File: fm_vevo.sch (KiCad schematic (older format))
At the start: 77 parts, among them J1 Bemenet, J2 RedPitaya_OSC, J3 12VDC, J4 RedPitaya_IN, J5 AudioJack2, Q1 mmbfj310, Q2 MMBT3904, Q3 MMBT3904, Q4 MMBT3904, Q5 MMBT3904, U1 LM358

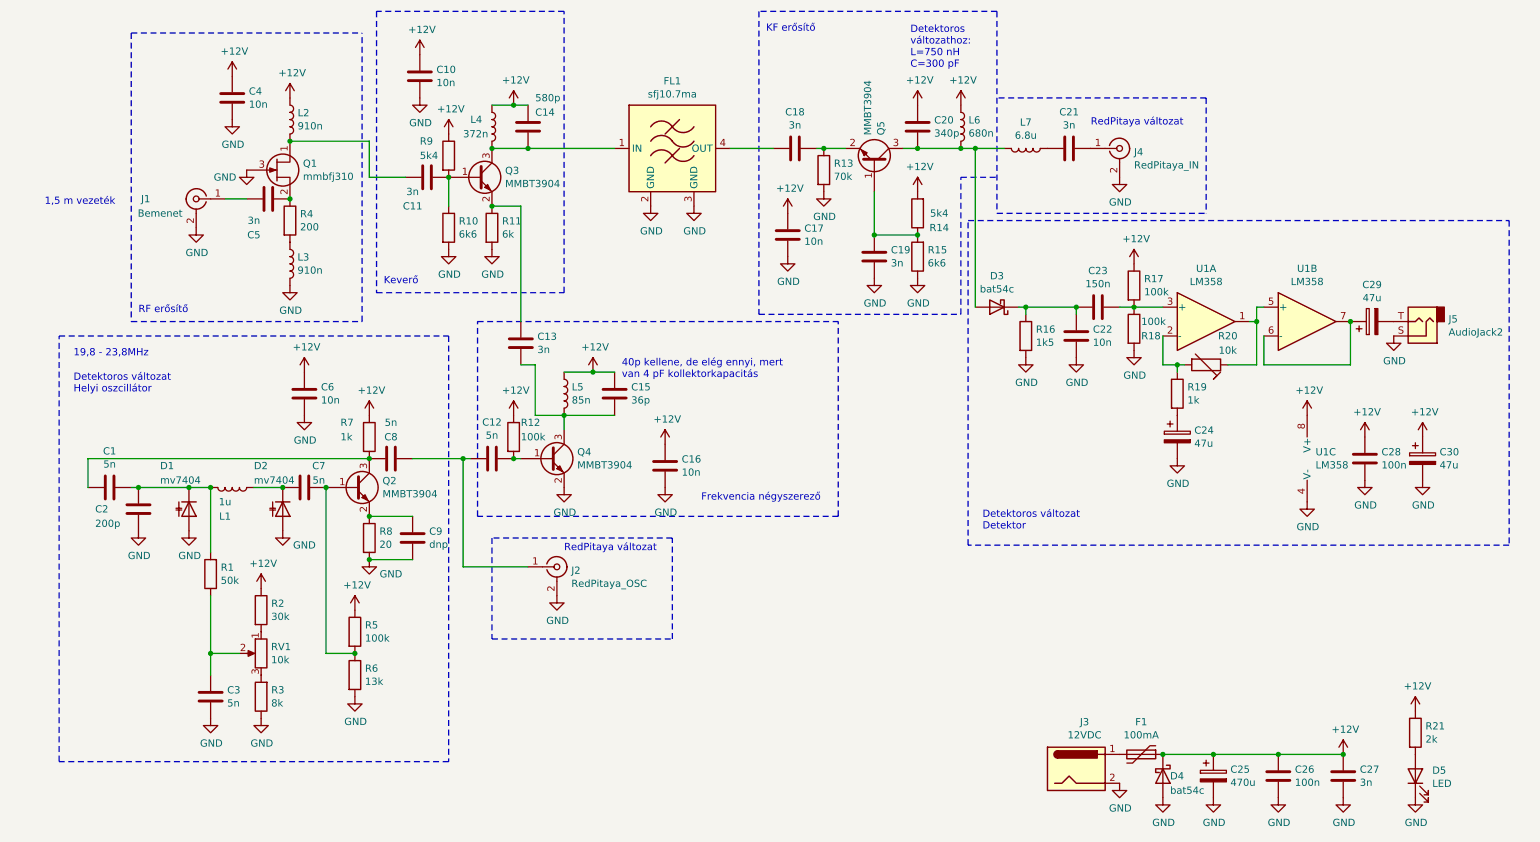
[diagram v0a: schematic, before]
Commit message: first sa612
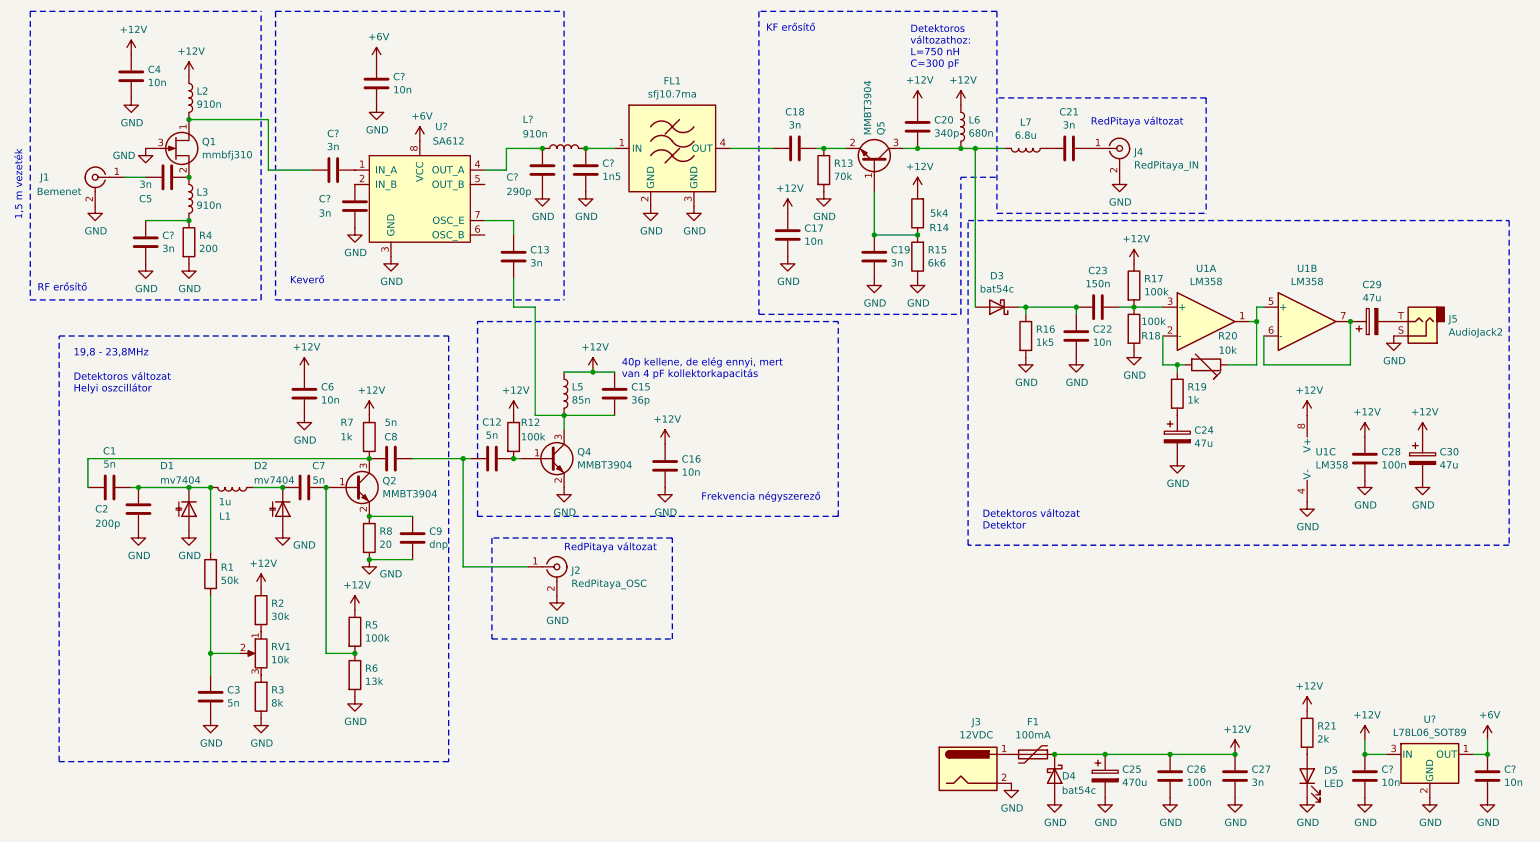
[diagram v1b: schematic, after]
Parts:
- removed C10: 10n, symbol Device:C
- removed C11: 3n, symbol Device:C
- removed C14: 580p, symbol Device:C
- removed L4: 372n, symbol Device:L
- removed Q3: MMBT3904, Package_TO_SOT_SMD:SOT-23, symbol Transistor_BJT:MMBT3904
- removed R10: 6k6, symbol Device:R
- removed R11: 6k, symbol Device:R
- removed R9: 5k4, symbol Device:R
- added C? (x3): 10n, symbol Device:C
- added C? (x3): 3n, symbol Device:C
- added C?: 290p, symbol Device:C
- added C?: 1n5, symbol Device:C
- added L?: 910n, symbol Device:L
- added U?: SA612, Package_SO:SO-8_3.9x4.9mm_P1.27mm, symbol custom:SA612
- added U?: L78L06_SOT89, Package_TO_SOT_SMD:SOT-89-3, symbol Regulator_Linear:L78L06_SOT89
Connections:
- net +12V: now also C?.1, U?.3 (IN)
- net GND: now also R4.2, C?.1, C?.2, C?.2, C?.2, C?.2, C?.2, C?.2, U?.2 (GND), U?.3 (GND); no longer L3.2
- net at C5.1, Q1.2 (S): now also L3.1; no longer R4.1
- net at L2.2, Q1.1 (D): now also C?.2
- net at FL1.1 (IN): now also C?.1, L?.2
- net at C13.1: now also U?.7 (OSC_E)
- new net: C?.1, L3.2, R4.1
- new net: C?.1, U?.1 (IN_A)
- new net: C?.2, U?.2 (IN_B)
- new net: C?.1, L?.1, U?.4 (OUT_A)
- new net +6V: C?.1, C?.1, U?.1 (OUT), U?.8 (VCC)
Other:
- moved on the sheet: C13, C25, C26, C27, C4, C5, D4, D5, F1, J1, J3, L2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
